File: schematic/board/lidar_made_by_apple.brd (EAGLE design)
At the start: 79.9 x 72.5 mm, 90 parts, among them J1 U.FL-R-SMT-1_10_, J2 U.FL-R-SMT-1_10_

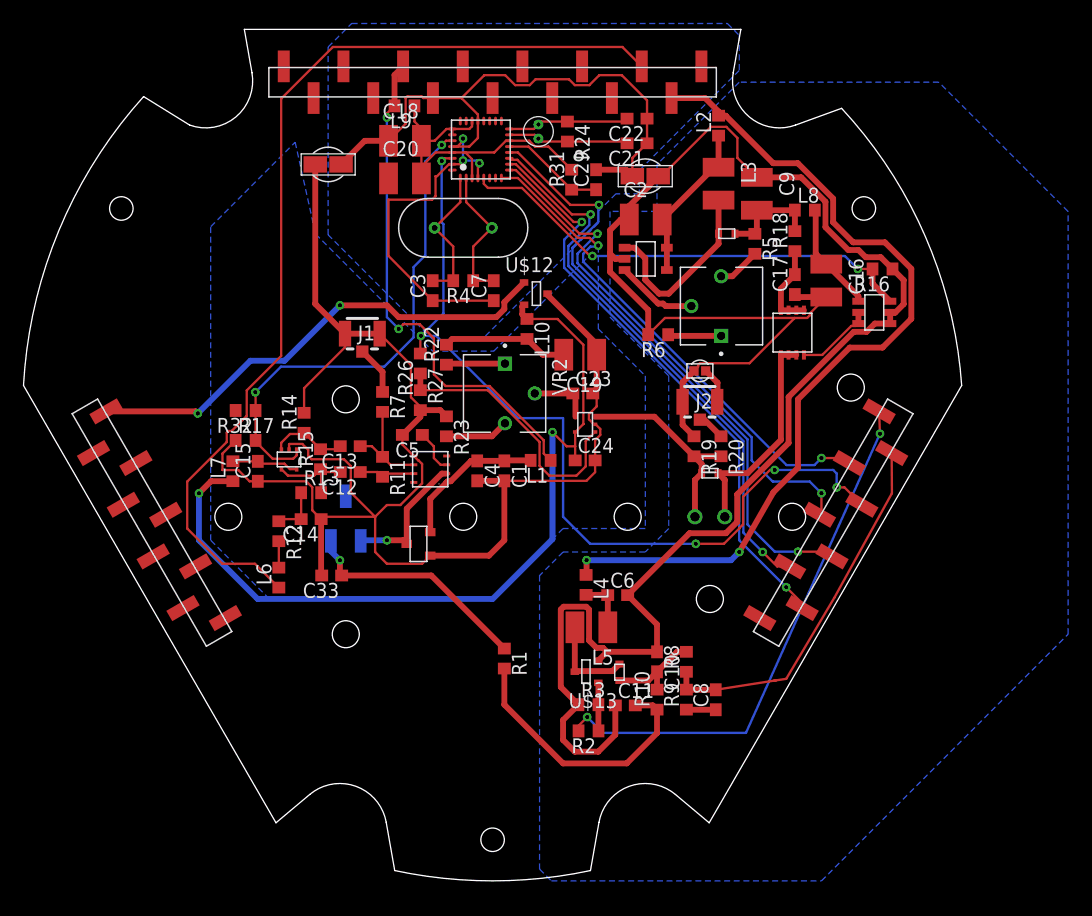
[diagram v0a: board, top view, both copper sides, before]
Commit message: ПЕРЕДЕЛАЙ ПАЛТЫ
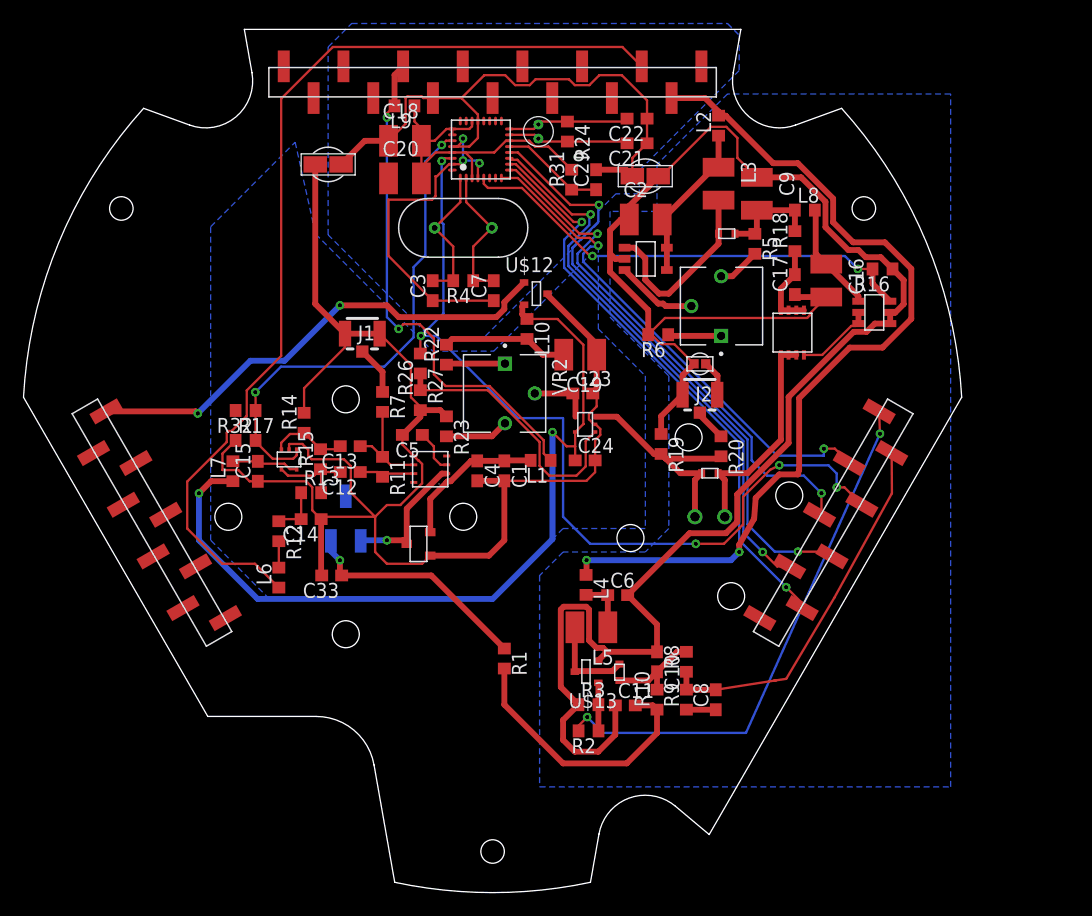
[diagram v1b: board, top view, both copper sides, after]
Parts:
- moved R19 2.81 mm to (64.3, 48.2)
- moved J2 0.60 mm to (67.7, 52.4)
- moved W3 0.60 mm to (67.7, 55.0)
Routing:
- net PGND: track 164.2 -> 158.9 mm
- net I_LASER: track 17.8 -> 20.4 mm
- net V_BAT: track 73.8 -> 74.9 mm
- net N$18: track 3.05 -> 3.65 mm
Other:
- board size 79.9 x 72.5 mm -> 79.9 x 73.5 mm
